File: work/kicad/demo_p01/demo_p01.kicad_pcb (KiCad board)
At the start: 2 copper layers, 2 parts

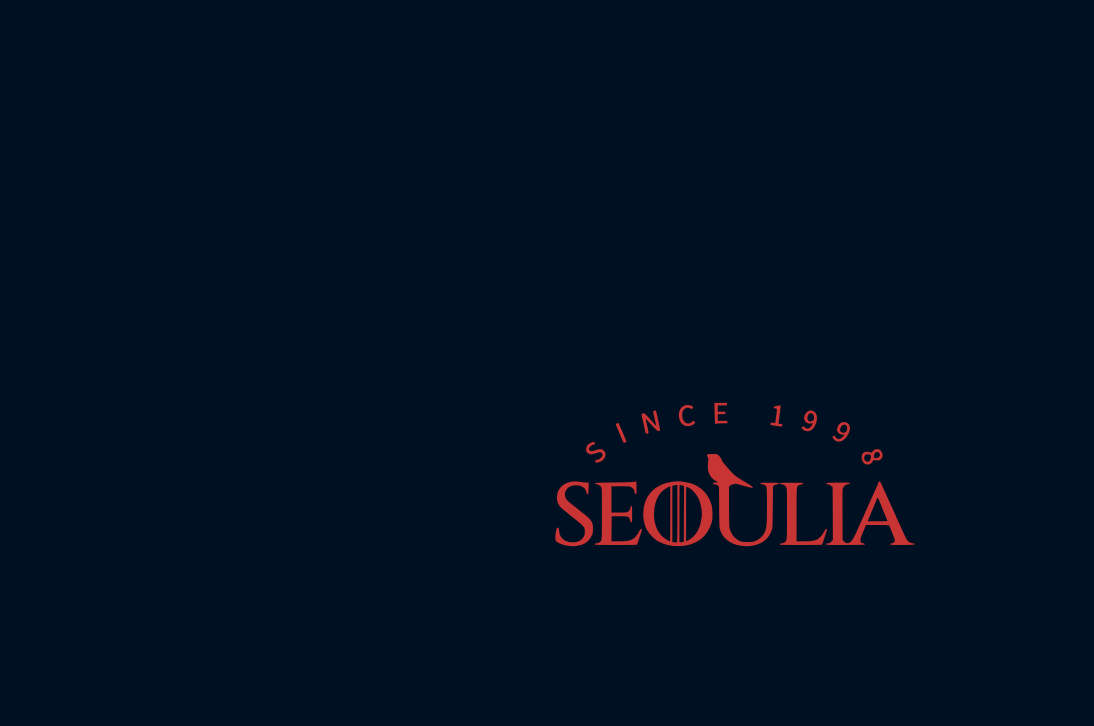
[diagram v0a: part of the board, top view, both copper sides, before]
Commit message: Arduino Study at 2022-08-26-[17:28]
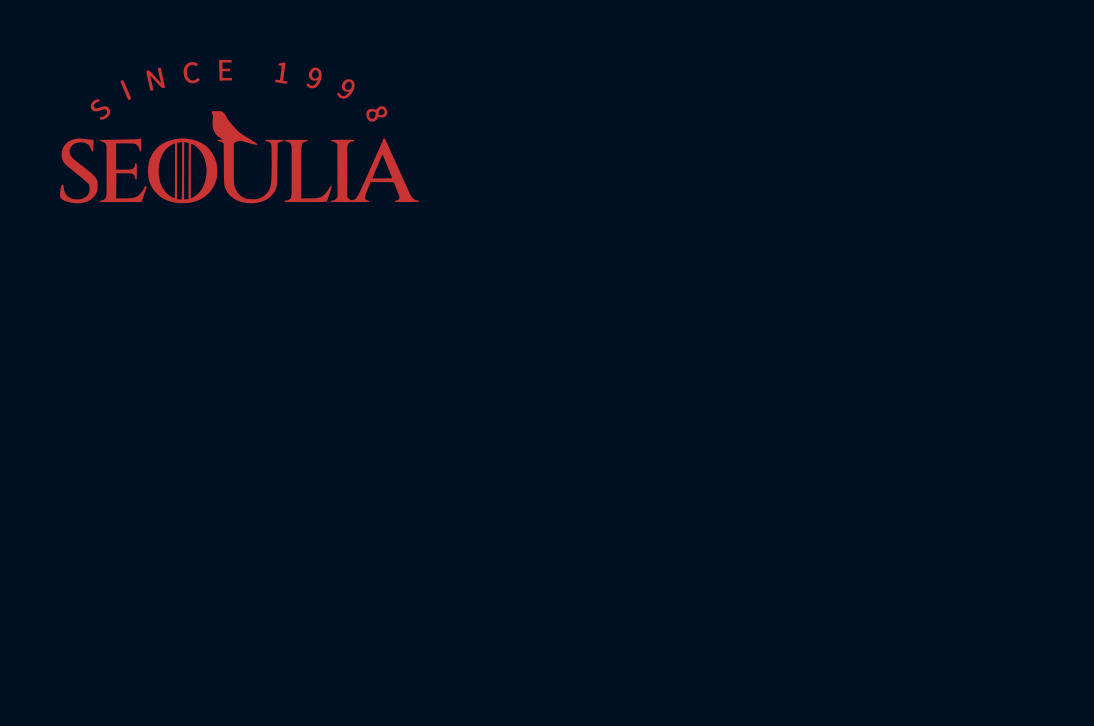
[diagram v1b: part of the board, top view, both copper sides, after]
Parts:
- moved G*** 20.1 mm to (163.8, 66.0)
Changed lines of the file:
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@@
   )
   (footprint "1_KJC_Library:KJC_logo_15" (layer "F.Cu")
-    (at 180.34 77.47)
+    (at 163.83 66.04)
     (attr board_only exclude_from_pos_files exclude_from_bom)
     (fp_text reference "G***" (at 20.955 -1.27) (layer "F.SilkS") hide
@@
       ) (layer "F.Cu") (width 0) (fill solid))
   )
+  (zone (net 0) (net_name "") (layer "F.Cu") (hatch edge 0.508)
+    (connect_pads (clearance 0))
+    (min_thickness 0.254)
+    (keepout (tracks not_allowed) (vias not_allowed) (pads not_allowed) (copperpour allowed) (footprints allowed))
+    (fill (thermal_gap 0.508) (thermal_bridge_width 0.508))
+    (polygon
+      (pts
+        (xy 218.44 87.63)
+        (xy 186.69 87.63)
+        (xy 186.69 53.34)
+        (xy 218.44 50.8)
+      )
+    )
+  )
 )
